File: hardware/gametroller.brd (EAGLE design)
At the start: 45.7 x 31.8 mm, 58 parts, among them J1 USB-MICRO, J2 PJ-002AH-SMT-TR, J3 USB-A, SW1 SPST_TACT-KMR2, U1 LP5907MFX-3.3/NOPB, U16 AOZ1280CI, U2 TPS2115AIPWRQ1-SON8, U4 ATSAMD21G18, X2 32.768

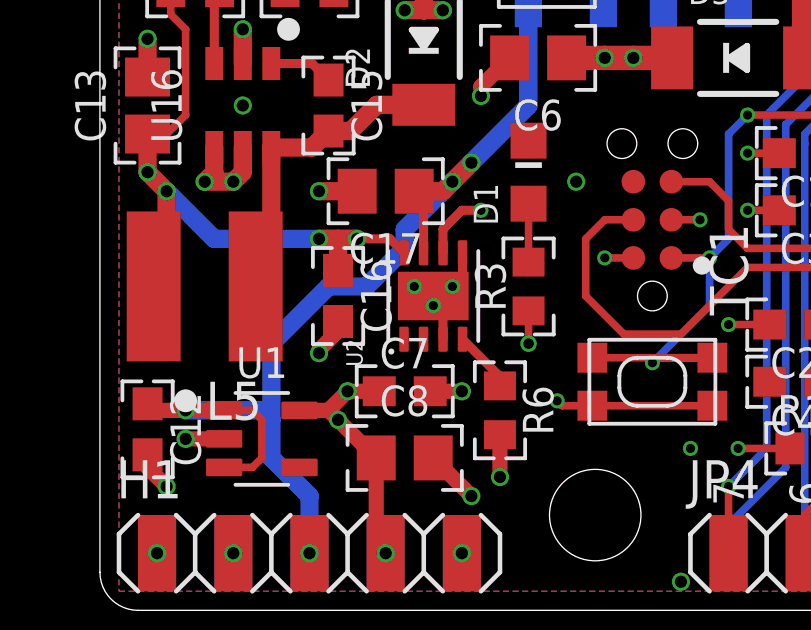
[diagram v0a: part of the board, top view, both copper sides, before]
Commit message: Minor hardware tweaks
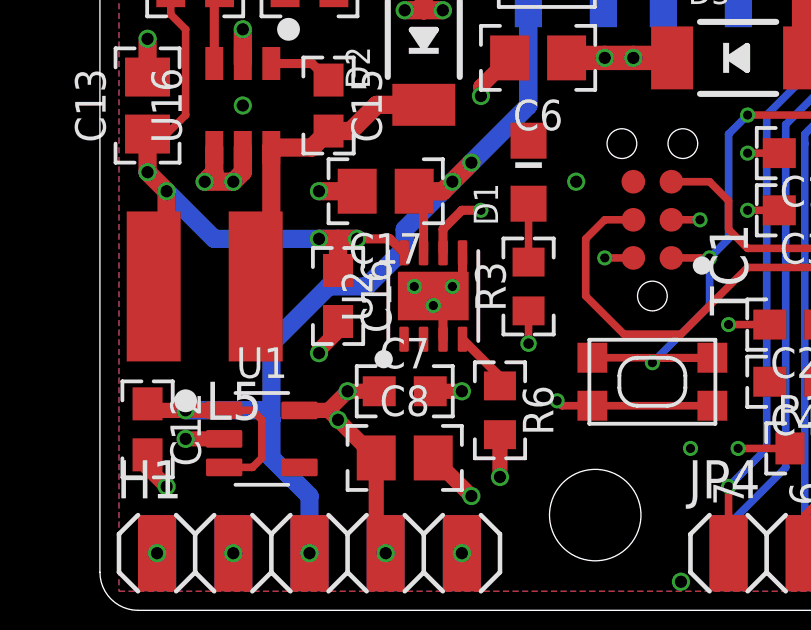
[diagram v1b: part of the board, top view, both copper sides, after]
